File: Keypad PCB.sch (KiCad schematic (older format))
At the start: 20 parts, among them J1 Conn_01x04_Female, SW1 SW_Push, U1 ATmega32U4-AU, Y1 Crystal_GND24_Small

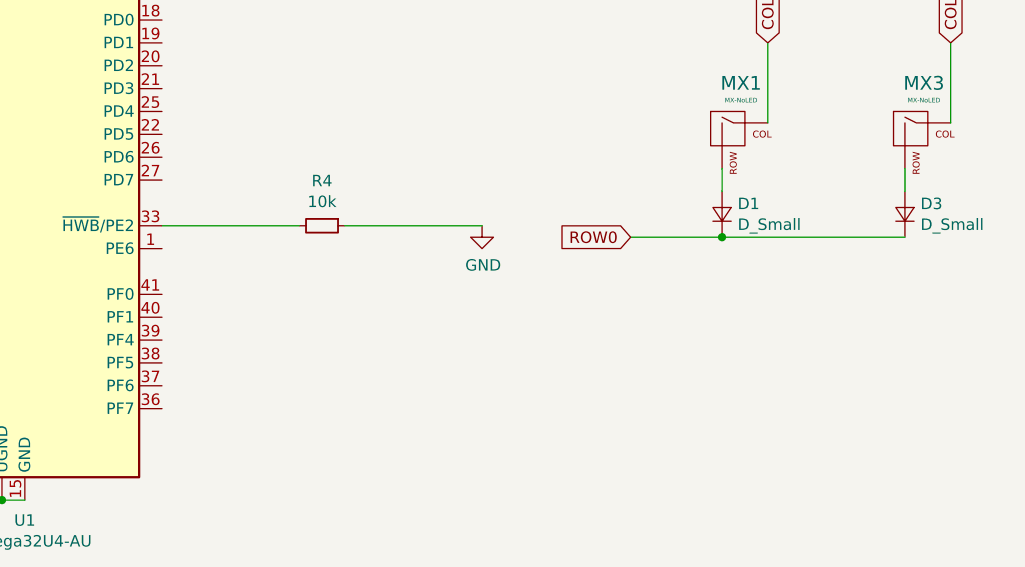
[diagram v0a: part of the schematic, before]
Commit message: OMG ?
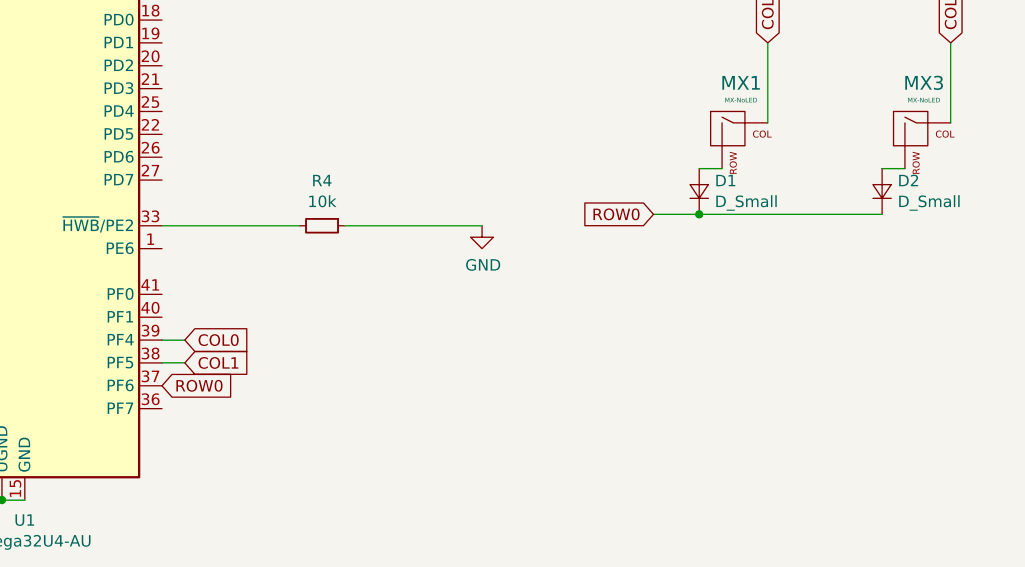
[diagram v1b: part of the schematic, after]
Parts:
- removed D3: D_Small, Diode_SMD:D_SOD-123, symbol Device:D_Small
- added D2: D_Small, Diode_SMD:D_SOD-123, symbol Device:D_Small
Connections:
- net COL0: now also U1.39 (PF4)
- net COL1: now also U1.38 (PF5)
- net ROW0: now also U1.37 (PF6), D2.1 (K)
- net at MX3.2 (ROW): now also D2.2 (A)
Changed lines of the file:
@@
 EESchema Schematic File Version 4
+LIBS:Keypad PCB-cache
 EELAYER 30 0
 EELAYER END
@@
 $EndDescr
 $Comp
-L MCU_Microchip_ATmega:ATmega32U4-AU U1
-U 1 1 63DFA3BE
-P 5500 3500
-F 0 "U1" H 5500 1611 50  0000 C CNN
-F 1 "ATmega32U4-AU" H 5500 1520 50  0000 C CNN
-F 2 "Package_QFP:TQFP-44_10x10mm_P0.8mm" H 5500 3500 50  0001 C CIN
-F 3 "http://ww1.microchip.com/downloads/en/DeviceDoc/Atmel-7766-8-bit-AVR-ATmega16U4-32U4_Datasheet.pdf" H 5500 3500 50  0001 C CNN
-	1    5500 3500
-	1    0    0    -1
-$EndComp
-$Comp
 L power:+5V #PWR0101
 U 1 1 63E012AE
@@
 Wire Wire Line
 	5400 1700 5400 1550
-Wire Wire Line
-	5400 1700 5500 1700
-Connection ~ 5400 1700
-Wire Wire Line
-	5500 1700 5600 1700
-Connection ~ 5500 1700
 $Comp
 L power:GND #PWR0102
@@
 	1    0    0    -1
 $EndComp
-Wire Wire Line
-	4950 5300 5400 5300
-Wire Wire Line
-	5400 5300 5500 5300
-Connection ~ 5400 5300
 $Comp
 L power:GND #PWR0103
@@
 $EndComp
 Wire Wire Line
-	6100 4100 6700 4100
-Wire Wire Line
 	6900 4100 7500 4100
 $Comp
@@
 	1    0    0    -1
 $EndComp
-Wire Wire Line
-	8550 3850 8550 3950
 $Comp
 L MX_Alps_Hybrid:MX-NoLED MX3
@@
 	1    0    0    -1
 $EndComp
-$Comp
-L Device:D_Small D1
-U 1 1 63E40E4C
-P 8550 4050
-F 0 "D1" V 8596 3982 50  0000 R CNN
-F 1 "D_Small" V 8505 3982 50  0000 R CNN
-F 2 "Diode_SMD:D_SOD-123" V 8550 4050 50  0001 C CNN
-F 3 "~" V 8550 4050 50  0001 C CNN
-	1    8550 4050
-	0    -1   -1   0
-$EndComp
 Wire Wire Line
 	8750 3650 8750 3300
 Wire Wire Line
 	9550 3650 9550 3300
-$Comp
-L Device:D_Small D3
-U 1 1 63E57EF8
-P 9350 4050
-F 0 "D3" V 9396 3982 50  0000 R CNN
-F 1 "D_Small" V 9305 3982 50  0000 R CNN
-F 2 "Diode_SMD:D_SOD-123" V 9350 4050 50  0001 C CNN
-F 3 "~" V 9350 4050 50  0001 C CNN
-	1    9350 4050
-	0    -1   -1   0
-$EndComp
-Wire Wire Line
-	9350 3850 9350 3950
-Wire Wire Line
-	9350 4150 8550 4150
-Wire Wire Line
-	8550 4150 8150 4150
-Connection ~ 8550 4150
 Text GLabel 8750 3300 1    50   Input ~ 0
 COL0
 Text GLabel 9550 3300 1    50   Input ~ 0
 COL1
-Text GLabel 8150 4150 0    50   Input ~ 0
-ROW0
 Wire Wire Line
 	3450 2500 3450 2650
@@
 	-1   0    0    1
 $EndComp
+Connection ~ 5400 5300
+Wire Wire Line
+	4950 5300 5400 5300
+Connection ~ 5500 1700
+Connection ~ 5400 1700
+Wire Wire Line
+	6100 4100 6700 4100
+Wire Wire Line
+	5500 1700 5600 1700
+Wire Wire Line
+	5400 5300 5500 5300
+Wire Wire Line
+	5400 1700 5500 1700
+Text GLabel 6200 4700 2    50   Input ~ 0
+COL1
+Text GLabel 6200 4600 2    50   Input ~ 0
+COL0
+$Comp
+L MCU_Microchip_ATmega:ATmega32U4-AU U1
+U 1 1 63DFA3BE
+P 5500 3500
+F 0 "U1" H 5500 1611 50  0000 C CNN
+F 1 "ATmega32U4-AU" H 5500 1520 50  0000 C CNN
+F 2 "Package_QFP:TQFP-44_10x10mm_P0.8mm" H 5500 3500 50  0001 C CIN
+F 3 "http://ww1.microchip.com/downloads/en/DeviceDoc/Atmel-7766-8-bit-AVR-ATmega16U4-32U4_Datasheet.pdf" H 5500 3500 50  0001 C CNN
+	1    5500 3500
+	1    0    0    -1
+$EndComp
+Wire Wire Line
+	6100 4600 6200 4600
+Wire Wire Line
+	6100 4700 6200 4700
+$Comp
+L Device:D_Small D1
+U 1 1 63E15488
+P 8450 3950
+F 0 "D1" V 8496 3882 50  0000 R CNN
+F 1 "D_Small" V 8405 3882 50  0000 R CNN
+F 2 "Diode_SMD:D_SOD-123" V 8450 3950 50  0001 C CNN
+F 3 "~" V 8450 3950 50  0001 C CNN
+	1    8450 3950
+	0    -1   -1   0
+$EndComp
+$Comp
+L Device:D_Small D2
+U 1 1 63E15EE0
+P 9250 3950
+F 0 "D2" V 9296 3882 50  0000 R CNN
+F 1 "D_Small" V 9205 3882 50  0000 R CNN
+F 2 "Diode_SMD:D_SOD-123" V 9250 3950 50  0001 C CNN
+F 3 "~" V 9250 3950 50  0001 C CNN
+	1    9250 3950
+	0    -1   -1   0
+$EndComp
+Wire Wire Line
+	8450 3850 8550 3850
+Wire Wire Line
+	9250 3850 9350 3850
+Wire Wire Line
+	8250 4050 8450 4050
+Connection ~ 8450 4050
+Wire Wire Line
+	8450 4050 9250 4050
+Text GLabel 8250 4050 0    50   Input ~ 0
+ROW0
+Text GLabel 6100 4800 2    50   Input ~ 0
+ROW0
 $EndSCHEMATC
